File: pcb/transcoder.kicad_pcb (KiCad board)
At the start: 2 copper layers, 74 x 41.8 mm, 35 parts, among them J1 MD-90SM, J2 Connector_RCA_2x3_REB, U1 BA7230LS, U2 LM1881, U3 THS7374

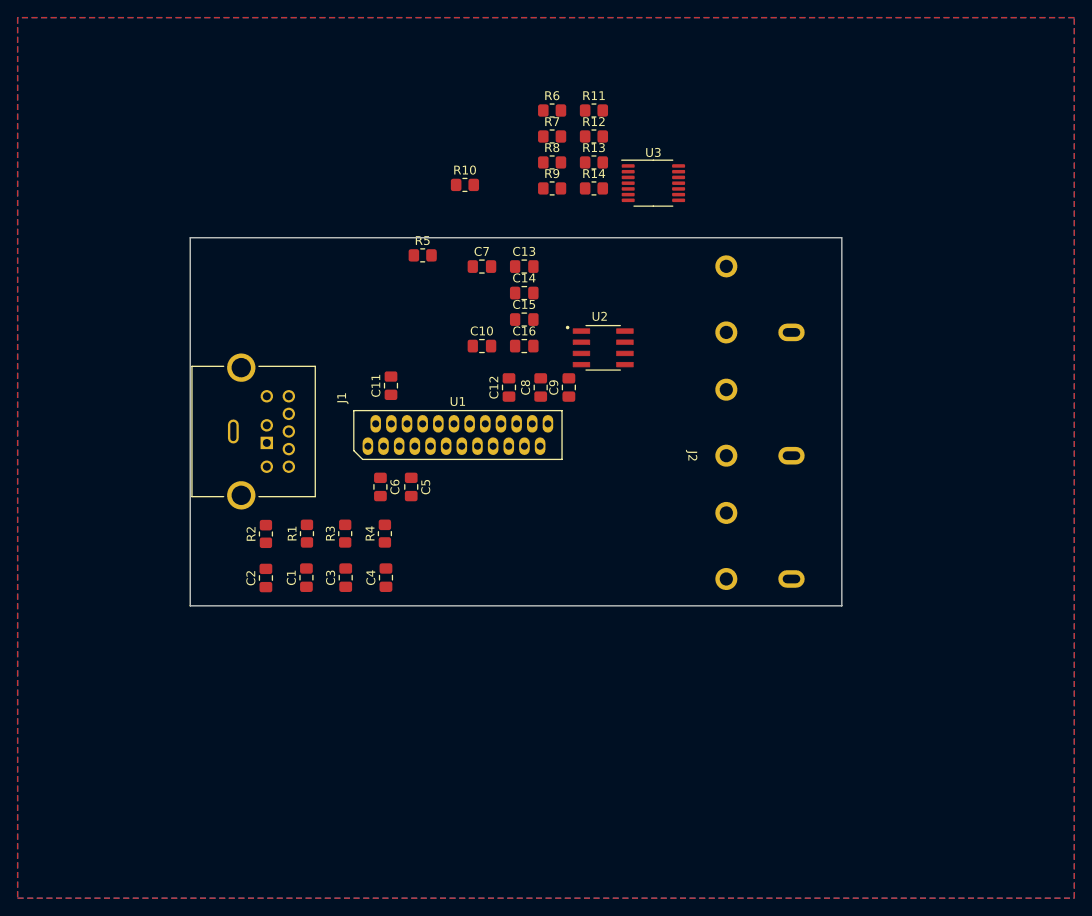
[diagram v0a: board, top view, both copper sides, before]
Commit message: Update
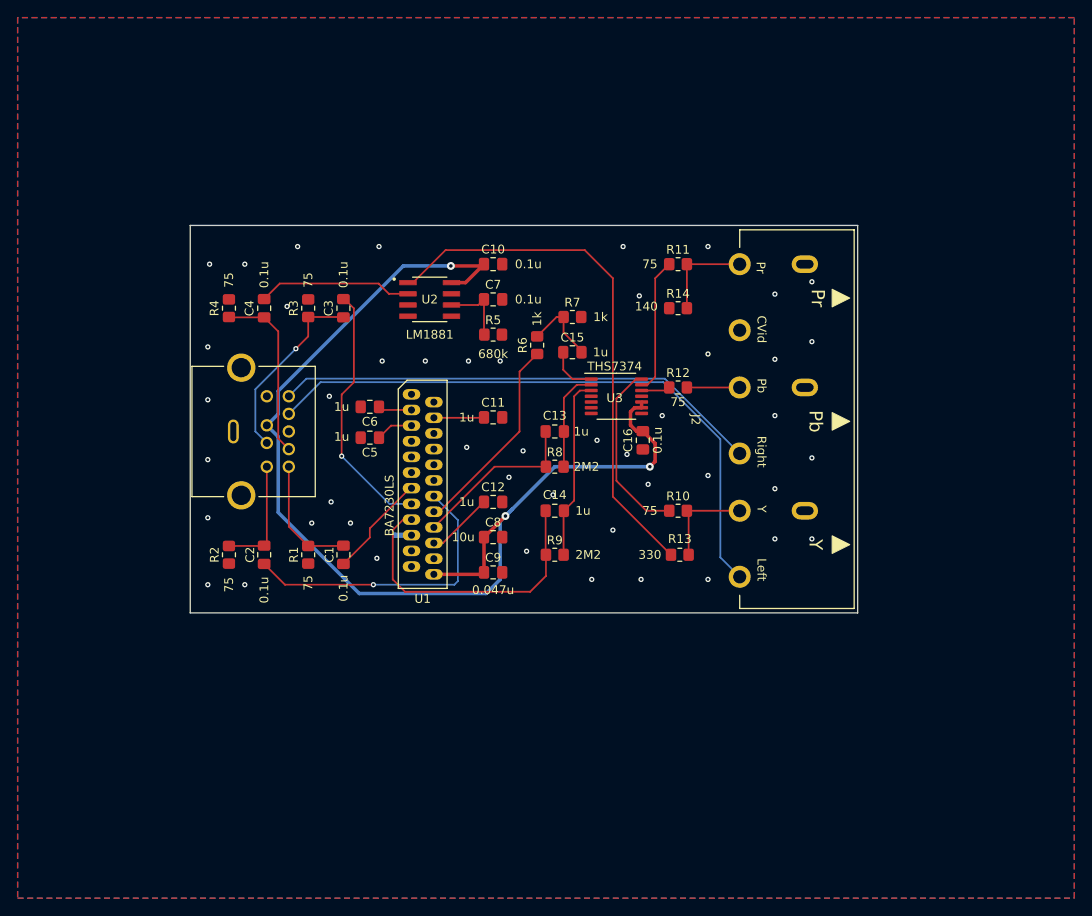
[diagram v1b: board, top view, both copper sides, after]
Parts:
- moved R13 45.6 mm to (175.2, 111.0), turned to 180 degrees
- moved R10 44.2 mm to (175.0, 106.0)
- moved R9 41.6 mm to (161.0, 111.0)
- moved R8 34.6 mm to (161.0, 101.0)
- moved C4 33.6 mm to (128.0, 83.0)
- moved R4 31.1 mm to (124.0, 83.0)
- moved C3 30.6 mm to (137.0, 83.0)
- moved R12 30.1 mm to (175.0, 92.0)
- moved R6 26.7 mm to (159.0, 87.2), turned to 90 degrees
- moved R3 25.9 mm to (133.0, 83.0)
- moved C14 25.0 mm to (161.0, 106.0), turned to 180 degrees
- moved U3 24.6 mm to (168.0, 93.0)
- moved C9 22.7 mm to (154.0, 113.0), turned to 0 degrees
- moved R7 20.6 mm to (163.0, 84.0)
- moved U2 20.5 mm to (146.8, 82.0)
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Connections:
- C1 pad 2: /R_IN -> /R
- C2 pad 2: /G_IN -> /G
- C3 pad 2: /B_IN -> /B
- C4 pad 2: /CVID_IN -> /CVID
- J2 pad 1: /Y_OUT -> /PR_OUT
- J2 pad 2: /PB_OUT -> unconnected-(J2-Composite-Pad2)
- J2 pad 3: /PR_OUT -> /PB_OUT
- J2 pad 4: /LAUD -> /RAUD
- J2 pad 5: /RAUD -> /Y_OUT
- J2 pad 6: unconnected-(J2-C-Pad6) -> /LAUD
- U1 pad 13: /R_IN -> /R
- U1 pad 14: /G_IN -> /G
- U1 pad 15: /B_IN -> /B
- U2 pad 2: /CVID_IN -> /CVID
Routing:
- net +5V: track 0.00 -> 129.1 mm, vias 0 -> 3
- net /LAUD: track 0.00 -> 69.7 mm
- net /CSYNC: track 0.00 -> 60.3 mm
- net /RAUD: track 0.00 -> 55.5 mm
- net /PB: track 0.00 -> 34.4 mm
- net /G: track 0.00 -> 33.9 mm, vias 0 -> 1
- net /B: track 0.00 -> 29.2 mm, vias 0 -> 1
- net /Y: track 0.00 -> 23.1 mm
- net /B_IN: track 0.00 -> 21.3 mm, vias 0 -> 1
- net Net-(U3-CH3_IN): track 0.00 -> 20.7 mm
- net Net-(U3-CH1_OUT): track 0.00 -> 20.5 mm
- net /CVID_IN: track 0.00 -> 20.1 mm
- net /PR: track 0.00 -> 19.6 mm
- net /CVID: track 0.00 -> 17.5 mm
- net Net-(U3-CH2_OUT): track 0.00 -> 15.4 mm
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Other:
- board size 74 x 41.8 mm -> 75.8 x 44 mm
